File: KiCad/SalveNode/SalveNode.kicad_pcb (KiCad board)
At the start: 2 copper layers, 41.5 x 31 mm, 21 parts, among them IC1 DS89C21TMX_NOPB, IC2 TMP75AQDGKRQ1, IC3 VEML7700-TR, J2 AVR-ISP-6, J3 691382040006, U1 ATmega328PB-A, Y2 16M

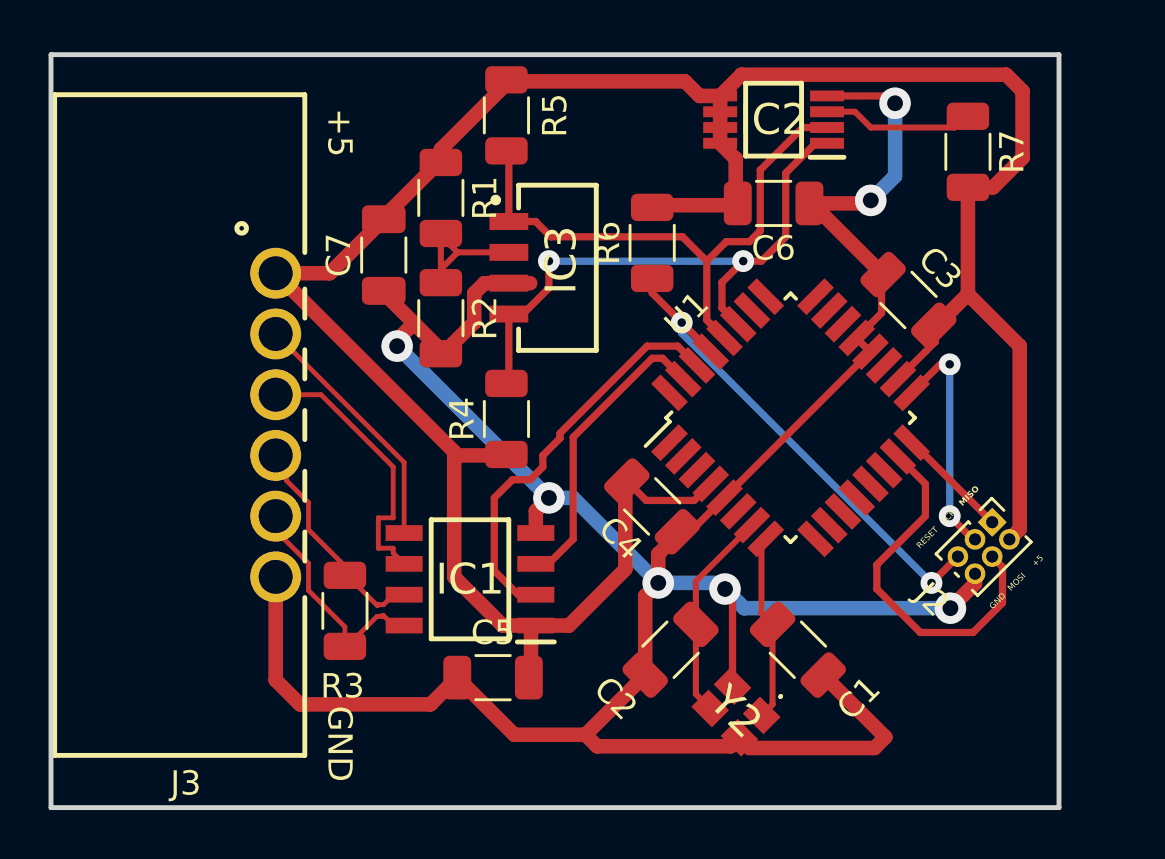
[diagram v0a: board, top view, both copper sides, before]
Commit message: Production
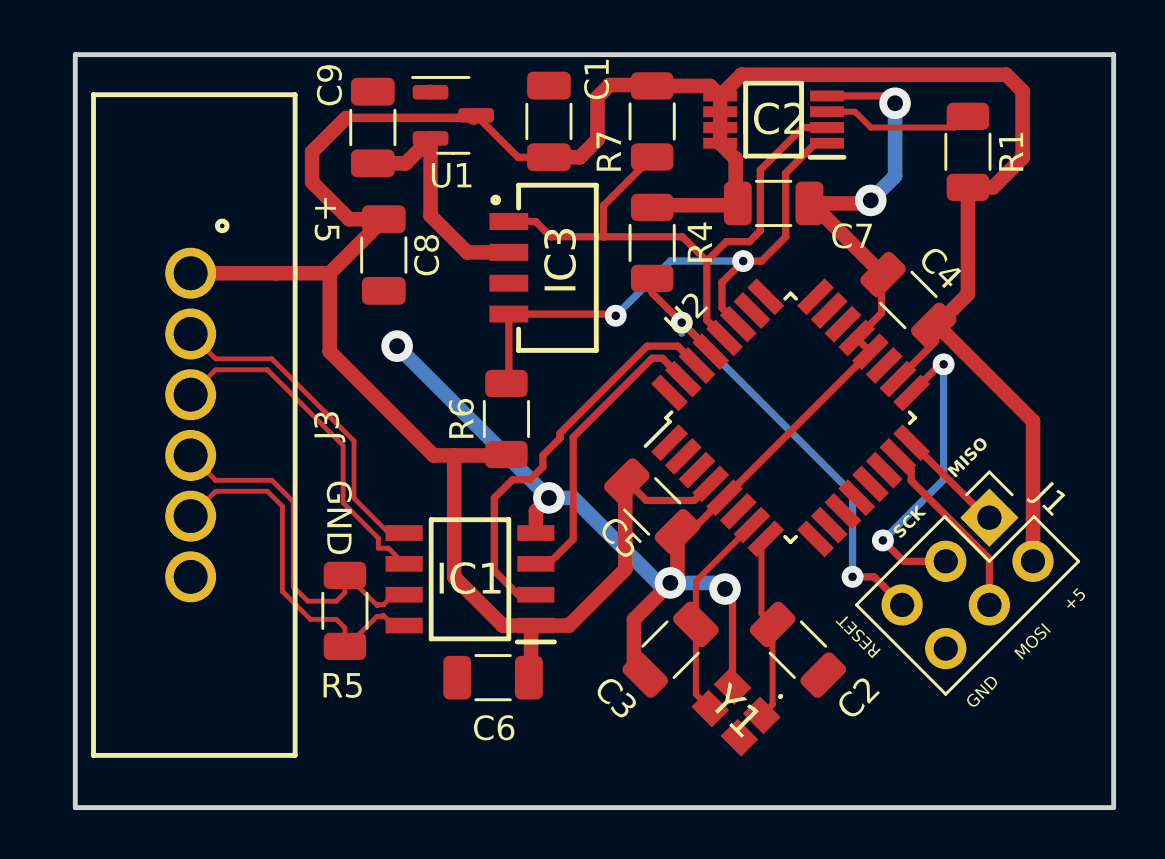
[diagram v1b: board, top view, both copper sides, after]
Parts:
- removed the R1 at (133.3, 45.9)
- removed R2: 2k, Resistor_SMD:R_1206_3216Metric
- added C1: 1u, Capacitor_SMD:C_1206_3216Metric, F.Cu at (137.8, 42.8)
- added C9: 1u, Capacitor_SMD:C_1206_3216Metric, F.Cu at (130.5, 43.0)
- added U1: MCP1700x-330xxTT, Package_TO_SOT_SMD:SOT-23, F.Cu at (133.8, 42.5)
- J1: renamed from J2; footprint Connector_PinHeader_1.00mm:PinHeader_2x03_P1.00mm_Vertical -> Connector_PinHeader_2.54mm:PinHeader_2x03_P2.54mm_Vertical
- J3: value 691382040006 -> 691382030006; footprint SimbolosSnapEDA:691382040006 -> SimbolosSnapEDA:691382030006
- R6: renamed from R4; value PAD -> 4.7k
- R7: renamed from R5; value PAD -> 4.7k
- moved R7 6.01 mm to (142.0, 42.8)
- moved J3 3.50 mm to (123.0, 55.2)
- moved J1 0.22 mm to (155.9, 59.1)
- renumbered C1 to C2, C2 to C3, C3 to C4, C4 to C5, C5 to C6, C6 to C7, C7 to C8, R7 to R1, R6 to R4, R3 to R5, U1 to U2, Y2 to Y1
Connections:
- IC3 pad 2: Net-(IC3-VDD) -> +3.3V
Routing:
- net Earth: track 120.1 -> 59.6 mm, vias 7 -> 6
- net +5V: track 105.7 -> 117.7 mm
- net +3.3V: track 0.00 -> 9.83 mm
- net /MOSI: track 15.3 -> 7.67 mm
- net Net-(IC3-VDD): track 6.38 -> 0.00 mm
- net /RI-: track 10.1 -> 16.1 mm
- net /RI+: track 10.2 -> 15.6 mm
- net /SCK: track 9.74 -> 13.0 mm
- net /D0-: track 10.4 -> 13.6 mm
- net /D0+: track 11.5 -> 14.1 mm
- net /SCL: track 24.5 -> 26.0 mm
- net /SDA: track 24.2 -> 23.6 mm
- added copper zone on F.Cu, net Earth
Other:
- board size 41.5 x 31 mm -> 42.8 x 31 mm
